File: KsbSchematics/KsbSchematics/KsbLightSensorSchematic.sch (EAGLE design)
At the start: 29 parts, among them IC1 7805L, IC2 LM311N, U1 ATTINY84

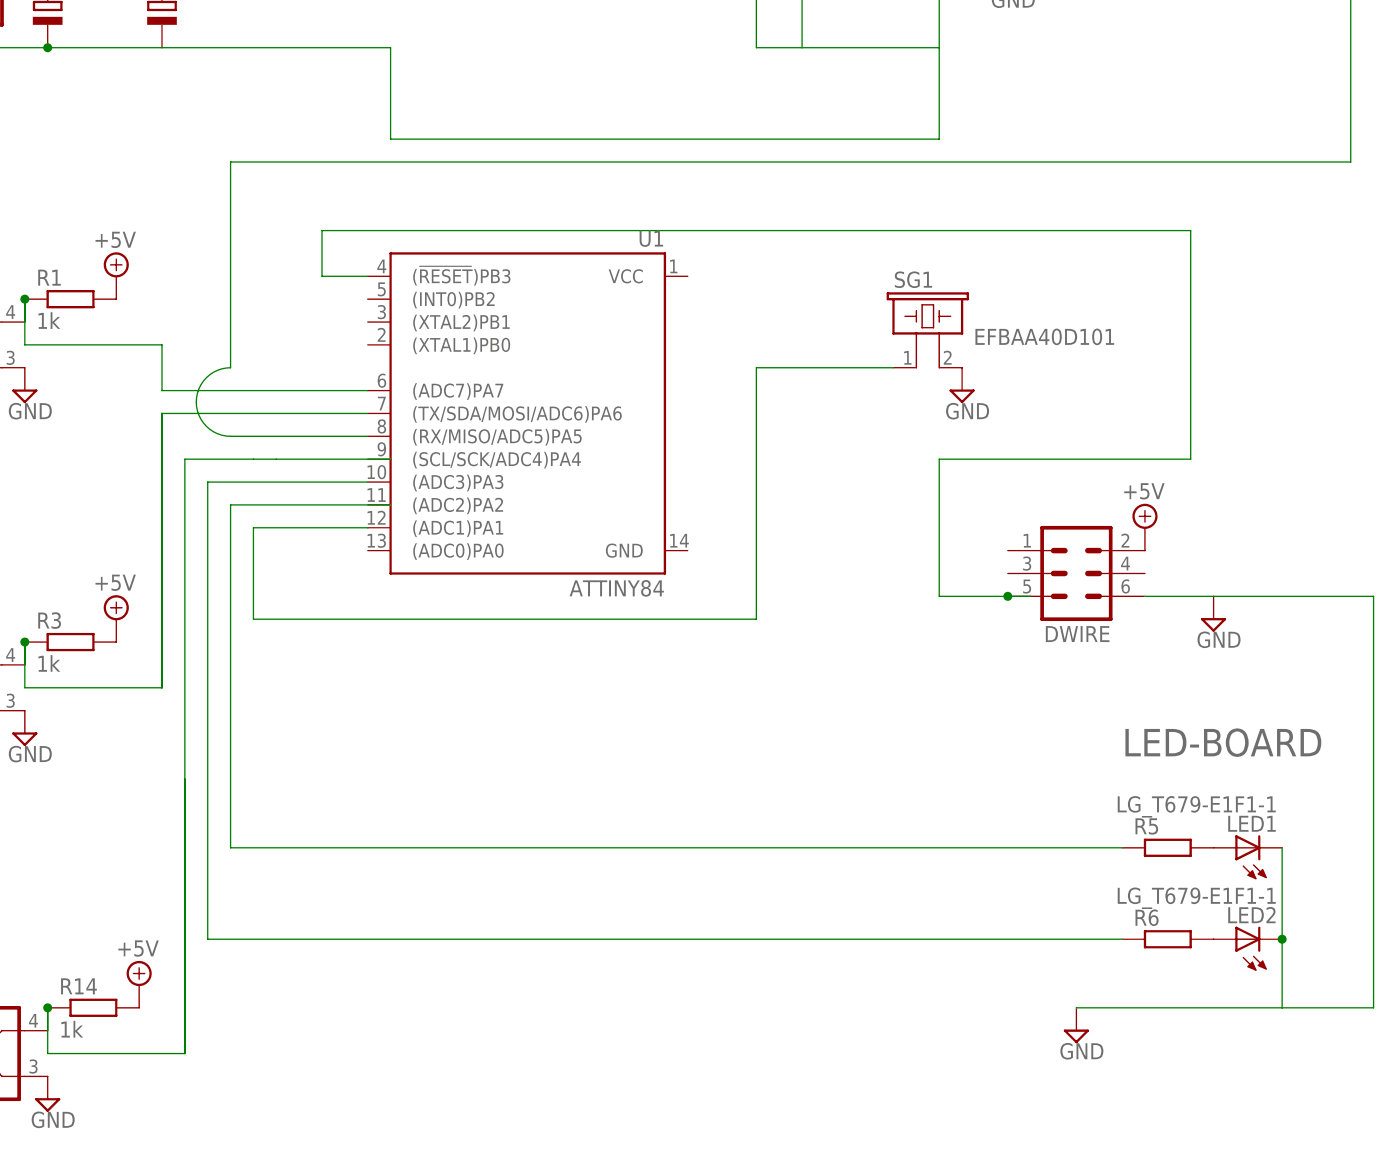
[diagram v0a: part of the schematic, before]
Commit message: schematic changes
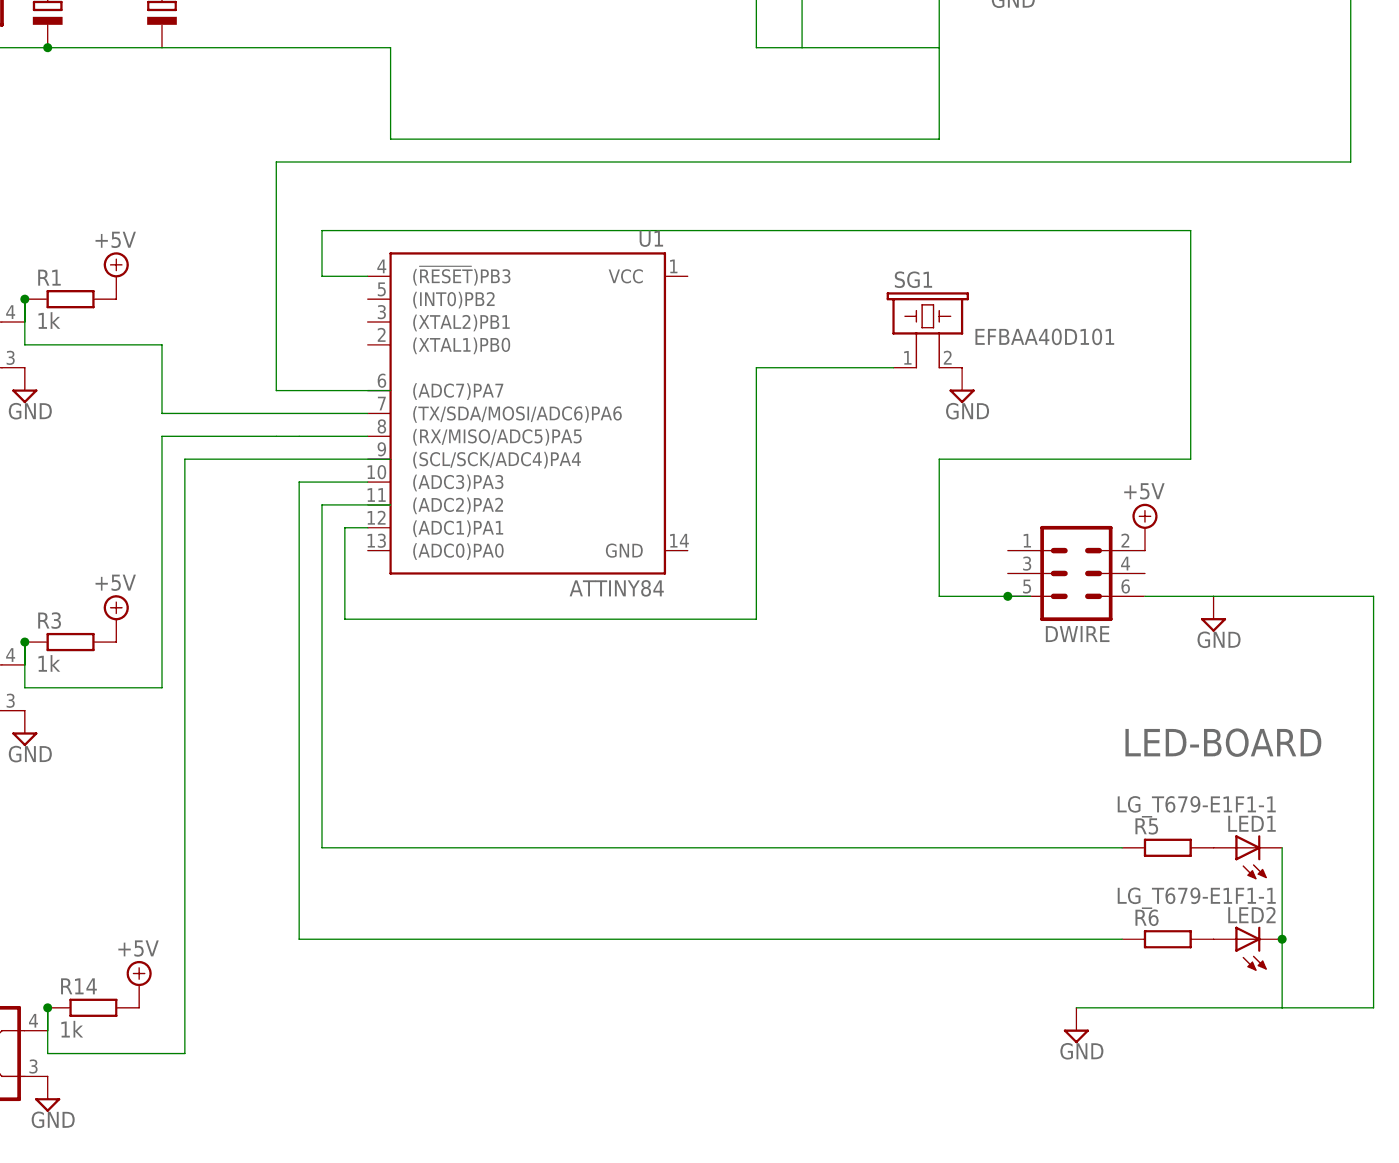
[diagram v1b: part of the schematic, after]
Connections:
- net N$15: now also U1.(TX/SDA/MOSI/ADC6)PA6; no longer U1.(ADC7)PA7
- net N$4: no longer U1.(RX/MISO/ADC5)PA5
- net N$6: now also U1.(RX/MISO/ADC5)PA5; no longer U1.(TX/SDA/MOSI/ADC6)PA6
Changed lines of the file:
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@@
 <rectangle x1="-30.48" y1="-5.08" x2="27.94" y2="154.94" layer="207"/>
 <polygon width="0.1524" layer="207">
-<vertex x="104.14" y="116.84"/>
+<vertex x="104.14" y="109.22"/>
 <vertex x="104.14" y="162.56"/>
 <vertex x="170.18" y="162.56"/>
 <vertex x="162.56" y="162.56"/>
 <vertex x="162.56" y="45.72"/>
-<vertex x="40.64" y="45.72"/>
-<vertex x="38.1" y="45.72"/>
-<vertex x="38.1" y="109.22"/>
-<vertex x="104.14" y="109.22"/>
-<vertex x="104.14" y="111.76"/>
+<vertex x="30.48" y="43.18"/>
+<vertex x="30.48" y="109.22"/>
 </polygon>
 <rectangle x1="111.76" y1="-2.54" x2="162.56" y2="35.56" layer="207"/>
@@
 <wire x1="7.62" y1="50.8" x2="7.62" y2="45.72" width="0.1524" layer="91"/>
 <wire x1="7.62" y1="45.72" x2="22.86" y2="45.72" width="0.1524" layer="91"/>
-<wire x1="22.86" y1="45.72" x2="22.86" y2="76.2" width="0.1524" layer="91"/>
-<wire x1="22.86" y1="76.2" x2="45.72" y2="76.2" width="0.1524" layer="91"/>
 <wire x1="7.62" y1="50.8" x2="7.62" y2="48.26" width="0.1524" layer="91"/>
 <junction x="7.62" y="50.8"/>
 <pinref part="OK4" gate="A" pin="COL"/>
 <pinref part="R3" gate="G$1" pin="1"/>
-<pinref part="U1" gate="U1" pin="(TX/SDA/MOSI/ADC6)PA6"/>
+<wire x1="22.86" y1="45.72" x2="22.86" y2="73.66" width="0.1524" layer="91"/>
+<pinref part="U1" gate="U1" pin="(RX/MISO/ADC5)PA5"/>
+<wire x1="45.72" y1="73.66" x2="38.1" y2="73.66" width="0.1524" layer="91"/>
+<wire x1="38.1" y1="73.66" x2="35.56" y2="73.66" width="0.1524" layer="91"/>
+<wire x1="22.86" y1="73.66" x2="35.56" y2="73.66" width="0.1524" layer="91"/>
 </segment>
 </net>
@@
 <net name="N$10" class="0">
 <segment>
-<wire x1="27.94" y1="68.58" x2="27.94" y2="17.78" width="0.1524" layer="91"/>
-<wire x1="27.94" y1="17.78" x2="129.54" y2="17.78" width="0.1524" layer="91"/>
+<wire x1="38.1" y1="68.58" x2="38.1" y2="17.78" width="0.1524" layer="91"/>
+<wire x1="38.1" y1="17.78" x2="129.54" y2="17.78" width="0.1524" layer="91"/>
 <pinref part="R6" gate="G$1" pin="1"/>
 <pinref part="U1" gate="U1" pin="(ADC3)PA3"/>
-<wire x1="27.94" y1="68.58" x2="45.72" y2="68.58" width="0.1524" layer="91"/>
-</segment>
-<segment>
-<wire x1="22.86" y1="76.2" x2="22.86" y2="45.72" width="0.1524" layer="91"/>
-</segment>
-<segment>
-<wire x1="22.86" y1="76.2" x2="22.86" y2="45.72" width="0.1524" layer="91"/>
+<wire x1="38.1" y1="68.58" x2="45.72" y2="68.58" width="0.1524" layer="91"/>
 </segment>
 </net>
 <net name="LED-BOARD" class="0">
 <segment>
-<wire x1="30.48" y1="66.04" x2="30.48" y2="27.94" width="0.1524" layer="91"/>
-<wire x1="30.48" y1="27.94" x2="129.54" y2="27.94" width="0.1524" layer="91"/>
+<wire x1="40.64" y1="66.04" x2="40.64" y2="27.94" width="0.1524" layer="91"/>
+<wire x1="40.64" y1="27.94" x2="129.54" y2="27.94" width="0.1524" layer="91"/>
 <pinref part="R5" gate="G$1" pin="1"/>
-<wire x1="30.48" y1="66.04" x2="48.26" y2="66.04" width="0.1524" layer="91"/>
+<wire x1="40.64" y1="66.04" x2="48.26" y2="66.04" width="0.1524" layer="91"/>
 <label x="129.54" y="38.1" size="3.048" layer="95"/>
 </segment>
@@
 <net name="N$4" class="0">
 <segment>
-<wire x1="30.48" y1="104.14" x2="30.48" y2="81.28" width="0.1524" layer="91"/>
-<wire x1="154.94" y1="104.14" x2="30.48" y2="104.14" width="0.1524" layer="91"/>
 <wire x1="154.94" y1="134.62" x2="154.94" y2="104.14" width="0.1524" layer="91"/>
 <wire x1="139.7" y1="134.62" x2="154.94" y2="134.62" width="0.1524" layer="91"/>
-<wire x1="30.48" y1="81.28" x2="30.48" y2="73.66" width="0.1524" layer="91" curve="180"/>
 <pinref part="IC2" gate="A" pin="OUT"/>
 <pinref part="R16" gate="G$1" pin="1"/>
 <junction x="154.94" y="134.62"/>
-<pinref part="U1" gate="U1" pin="(RX/MISO/ADC5)PA5"/>
-<wire x1="30.48" y1="73.66" x2="45.72" y2="73.66" width="0.1524" layer="91"/>
+<wire x1="154.94" y1="104.14" x2="35.56" y2="104.14" width="0.1524" layer="91"/>
+<wire x1="35.56" y1="104.14" x2="35.56" y2="78.74" width="0.1524" layer="91"/>
+<wire x1="35.56" y1="78.74" x2="48.26" y2="78.74" width="0.1524" layer="91"/>
 </segment>
 </net>
@@
 <segment>
 <wire x1="7.62" y1="88.9" x2="7.62" y2="83.82" width="0.1524" layer="91"/>
-<wire x1="45.72" y1="78.74" x2="22.86" y2="78.74" width="0.1524" layer="91"/>
-<wire x1="22.86" y1="78.74" x2="22.86" y2="83.82" width="0.1524" layer="91"/>
 <wire x1="22.86" y1="83.82" x2="7.62" y2="83.82" width="0.1524" layer="91"/>
 <wire x1="7.62" y1="88.9" x2="7.62" y2="86.36" width="0.1524" layer="91"/>
@@
 <pinref part="OK3" gate="A" pin="COL"/>
 <pinref part="R1" gate="G$1" pin="1"/>
-<pinref part="U1" gate="U1" pin="(ADC7)PA7"/>
+<wire x1="22.86" y1="83.82" x2="22.86" y2="76.2" width="0.1524" layer="91"/>
+<pinref part="U1" gate="U1" pin="(TX/SDA/MOSI/ADC6)PA6"/>
+<wire x1="22.86" y1="76.2" x2="45.72" y2="76.2" width="0.1524" layer="91"/>
 </segment>
 </net>
@@
 <pinref part="R14" gate="G$1" pin="1"/>
 <wire x1="25.4" y1="5.08" x2="25.4" y2="71.12" width="0.1524" layer="91"/>
-<wire x1="25.4" y1="71.12" x2="33.02" y2="71.12" width="0.1524" layer="91"/>
-<wire x1="33.02" y1="71.12" x2="35.56" y2="71.12" width="0.1524" layer="91"/>
-<wire x1="35.56" y1="71.12" x2="48.26" y2="71.12" width="0.1524" layer="91"/>
-</segment>
-</net>
-<net name="N$12" class="0">
-<segment>
-<wire x1="25.4" y1="35.56" x2="25.4" y2="5.08" width="0.1524" layer="91"/>
-</segment>
-<segment>
-<wire x1="25.4" y1="35.56" x2="25.4" y2="5.08" width="0.1524" layer="91"/>
+<wire x1="25.4" y1="71.12" x2="48.26" y2="71.12" width="0.1524" layer="91"/>
 </segment>
 </net>
@@
 <wire x1="104.14" y1="81.28" x2="88.9" y2="81.28" width="0.1524" layer="91"/>
 <wire x1="88.9" y1="81.28" x2="88.9" y2="53.34" width="0.1524" layer="91"/>
-<wire x1="88.9" y1="53.34" x2="33.02" y2="53.34" width="0.1524" layer="91"/>
-<wire x1="33.02" y1="53.34" x2="33.02" y2="63.5" width="0.1524" layer="91"/>
+<wire x1="88.9" y1="53.34" x2="43.18" y2="53.34" width="0.1524" layer="91"/>
+<wire x1="43.18" y1="53.34" x2="43.18" y2="63.5" width="0.1524" layer="91"/>
 <pinref part="U1" gate="U1" pin="(ADC1)PA1"/>
-<wire x1="33.02" y1="63.5" x2="45.72" y2="63.5" width="0.1524" layer="91"/>
-</segment>
-</net>
+<wire x1="43.18" y1="63.5" x2="45.72" y2="63.5" width="0.1524" layer="91"/>
+</segment>
+</net>
